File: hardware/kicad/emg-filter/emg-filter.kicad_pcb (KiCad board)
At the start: 4 copper layers, 50 x 40 mm, 84 parts, among them J1 Conn_01x02, J10 Conn_01x02, J11 Conn_01x02, J2 Conn_01x05, J3 Conn_01x02, J4 Conn_01x02, J5 Conn_01x02, J6 Conn_01x02, J7 Conn_01x02, J8 Conn_01x02, J9 Conn_01x02, U1 LM4565, U2 LM4565, U3 LM4565, U4 LM4565, U5 LM4565, U6 LM4565, U7 INA2332

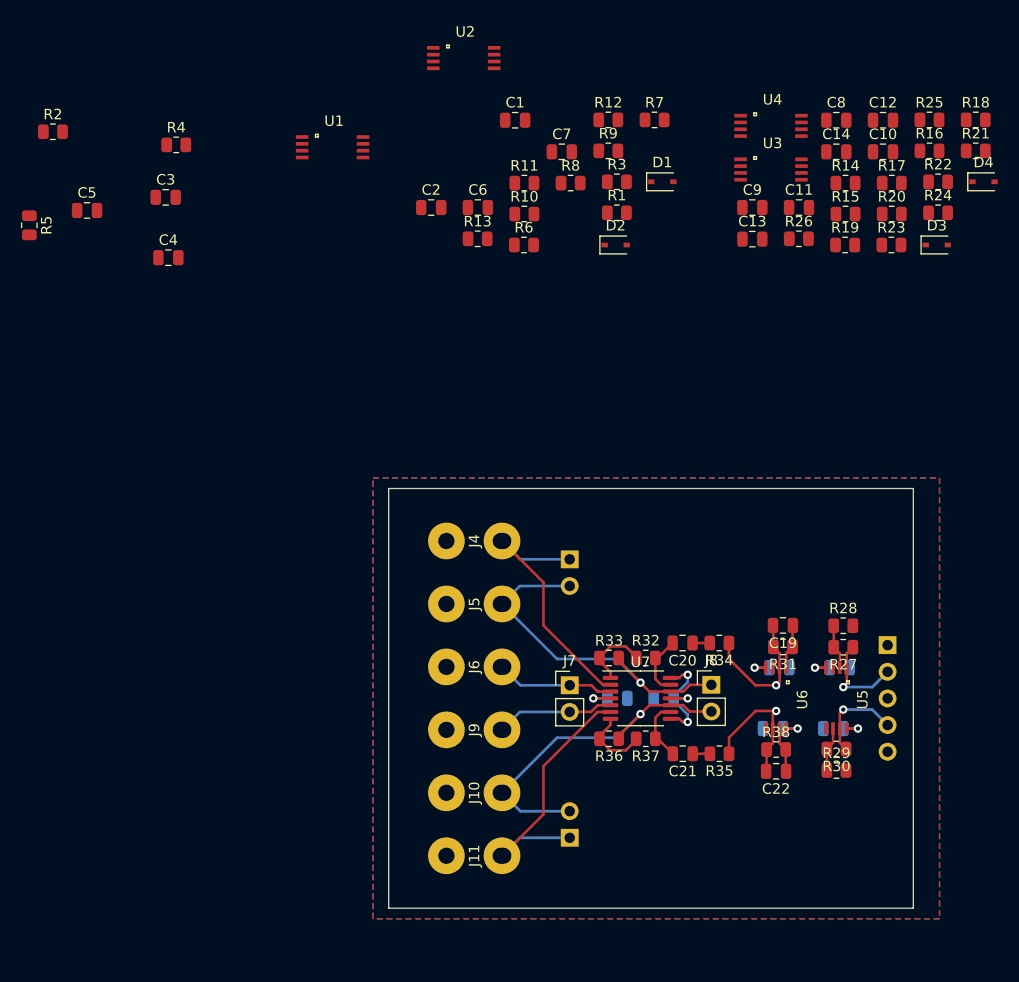
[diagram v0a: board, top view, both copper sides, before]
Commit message: Done - Ready for manufacturing
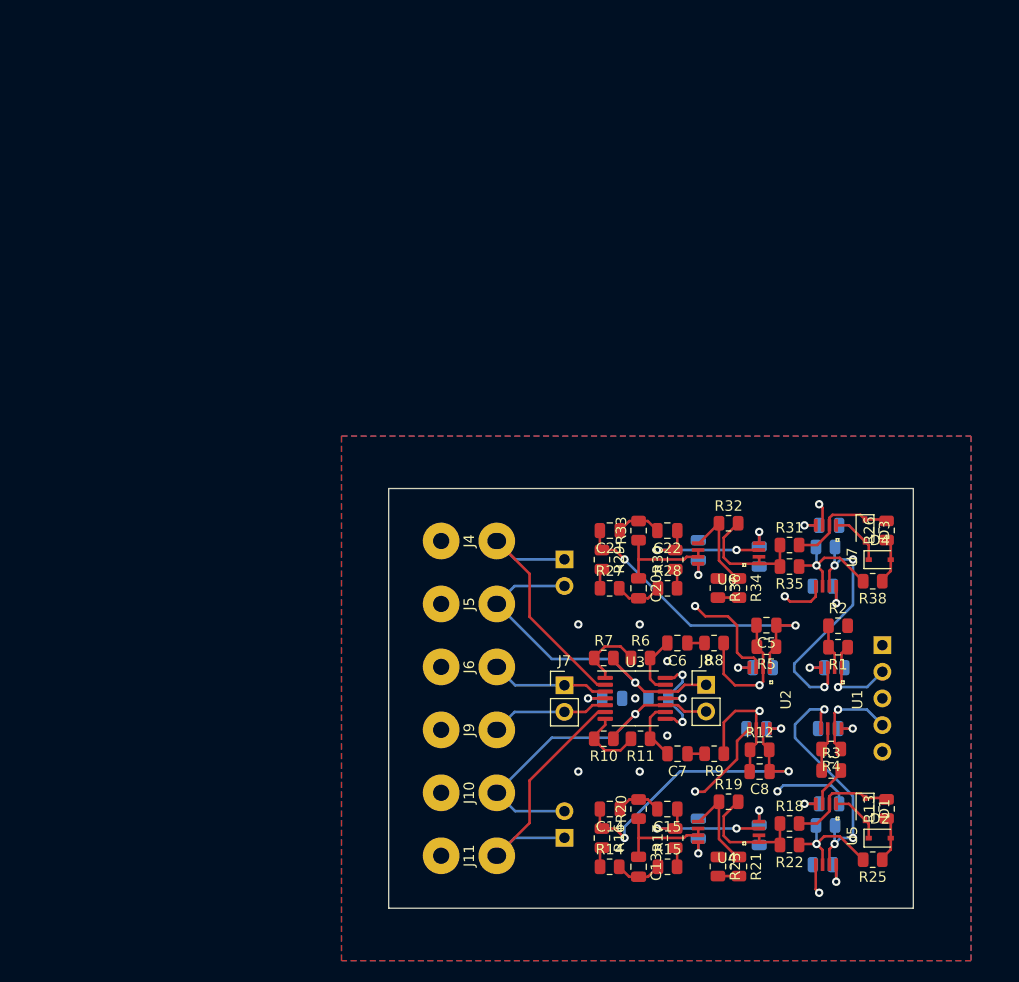
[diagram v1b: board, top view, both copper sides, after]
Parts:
- C1, C2, C9: moved to B.Cu
- C10, C3: value 20n -> 0.1u; moved to B.Cu
- C11, C12, C4: value 10n -> 0.1u; moved to B.Cu
- C13, C6, C7: value 0.1u -> 20n
- C14: value 0.1u -> 10n
- C15: value 0.1u -> 10n; moved to F.Cu
- C19: value 2n -> 0.1u; moved to B.Cu
- C21: value 20n -> 10n
- C22: value 2n -> 10n
- C5: value 10n -> 2n
- C8: value 0.1u -> 2n
- R11: value 133k -> 191k
- R12: value 10k -> 261k
- R13, R26: value 5k -> 10k
- R14, R27: value 10k -> 132k
- R15, R17: value 132k -> 133k
- R16: value 133k -> 132k
- R18, R22: value 133k -> 10k
- R19: value 10k -> 2k
- R2: value 132k -> 2k
- R20, R28: value 2k -> 133k
- R23, R30, R33, R36: value 10k -> 133k
- R24: value 133k -> 10k; moved to B.Cu
- R25: value 10k -> 5k
- R29: value 2k -> 132k
- R3: value 133k -> 2k
- R31, R35: value 261k -> 10k
- R32: value 191k -> 2k
- R34: value 261k -> 133k
- R37: value 191k -> 10k; moved to B.Cu
- R38: value 261k -> 5k
- R4: value 132k -> 10k
- R5, R8, R9: value 133k -> 261k
- R6: value 10k -> 191k
- R7: value 2k -> 10k
- U3: value LM4565 -> INA2332; footprint emg-filter:LM4565 -> Package_SO:TSSOP-14_4.4x5mm_P0.65mm
- U7: value INA2332 -> LM4565; footprint Package_SO:TSSOP-14_4.4x5mm_P0.65mm -> emg-filter:LM4565
- moved R2 88.4 mm to (92.3, 108.1)
- moved R4 84.9 mm to (91.7, 119.8), turned to 180 degrees
- moved R5 80.9 mm to (85.5, 110.1), turned to 180 degrees
- moved C5 75.9 mm to (85.5, 108.0), turned to 180 degrees
- moved R16 72.6 mm to (69.8, 128.3), turned to 270 degrees
- moved U1 72.1 mm to (92.7, 112.1), turned to 270 degrees
- moved R21 71.8 mm to (82.9, 131.0), turned to 270 degrees
- moved C4 71.8 mm to (84.5, 117.9), turned to 180 degrees
- moved C12 71.2 mm to (90.9, 130.8), turned to 180 degrees
- moved R25 70.7 mm to (95.6, 130.4), turned to 180 degrees
- moved R18 69.4 mm to (87.7, 126.9)
- moved U4 69.3 mm to (84.8, 128.7), turned to 180 degrees
- moved R14 68.9 mm to (70.6, 131.1)
- moved U2 67.2 mm to (85.8, 112.1), turned to 270 degrees
- moved C3 67.0 mm to (75.2, 115.0)
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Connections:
- C1 pad 1: +5V -> GND
- C1 pad 2: GND -> +5V
- C10 pad 1: Net-(C10-Pad1) -> GND
- C10 pad 2: Net-(C10-Pad2) -> -5V
- C11 pad 1: Net-(C11-Pad1) -> +5V
- C11 pad 2: /emg_module/sheet625420FA/BP_NOTCH -> GND
- C12 pad 1: Net-(C12-Pad1) -> +5V
- C12 pad 2: Net-(C11-Pad1) -> GND
- C13 pad 1: GND -> Net-(C13-Pad1)
- C13 pad 2: -5V -> Net-(C13-Pad2)
- C14 pad 1: -5V -> Net-(C14-Pad1)
- C14 pad 2: GND -> /emg_module/sheet625420F9/BP_NOTCH
- C15 pad 1: GND -> Net-(C15-Pad1)
- C15 pad 2: +5V -> Net-(C14-Pad1)
- C16 pad 1: -5V -> GND
- C16 pad 2: GND -> -5V
- C17 pad 1: GND -> -5V
- C17 pad 2: +5V -> GND
- C19 pad 1: /emg_module/sheet625420FA/BP_NOTCH -> +5V
- C19 pad 2: Net-(C19-Pad2) -> GND
- C2 pad 1: +5V -> -5V
- C21 pad 2: Net-(C21-Pad2) -> /emg_module/sheet625420FA/BP_NOTCH
- C22 pad 1: /emg_module/sheet625420F9/BP_NOTCH -> Net-(C22-Pad1)
- C22 pad 2: Net-(C22-Pad2) -> Net-(C21-Pad1)
- C24 pad 1: GND -> -5V
- C24 pad 2: -5V -> GND
- C3 pad 1: Net-(C3-Pad1) -> GND
- C3 pad 2: Net-(C3-Pad2) -> +5V
- C4 pad 1: Net-(C4-Pad1) -> +5V
- C4 pad 2: /emg_module/sheet625420F9/BP_NOTCH -> GND
- C5 pad 1: Net-(C5-Pad1) -> /emg_module/sheet625420FA/BP_NOTCH
- C5 pad 2: Net-(C4-Pad1) -> Net-(C5-Pad2)
- C6 pad 1: GND -> Net-(C6-Pad1)
- C6 pad 2: -5V -> Net-(C6-Pad2)
- C7 pad 1: -5V -> Net-(C7-Pad1)
- C7 pad 2: GND -> Net-(C7-Pad2)
- C8 pad 1: +5V -> /emg_module/sheet625420F9/BP_NOTCH
- C8 pad 2: GND -> Net-(C8-Pad2)
- C9 pad 1: +5V -> GND
- C9 pad 2: GND -> -5V
- R1 pad 1: Net-(D2-Pad2) -> /emg_module/OUT_A
- R1 pad 2: Net-(D1-Pad1) -> Net-(R1-Pad2)
- R10 pad 1: Net-(R10-Pad1) -> /emg_module/REF_B
- R11 pad 1: GND -> Net-(C7-Pad2)
- R11 pad 2: Net-(R11-Pad2) -> Net-(R10-Pad2)
- R12 pad 1: /emg_module/sheet625420F9/RECT_AMP -> Net-(C8-Pad2)
- R12 pad 2: Net-(R10-Pad1) -> /emg_module/sheet625420F9/BP_NOTCH
- R13 pad 2: Net-(R10-Pad1) -> Net-(D1-Pad1)
- R14 pad 1: Net-(D4-Pad2) -> Net-(R14-Pad1)
- R14 pad 2: Net-(D3-Pad1) -> Net-(C13-Pad2)
- R15 pad 1: Net-(R15-Pad1) -> Net-(C13-Pad2)
- R15 pad 2: Net-(C10-Pad2) -> Net-(R15-Pad2)
- R16 pad 1: Net-(C10-Pad2) -> /emg_module/sheet625420F9/BP_NOTCH
- R16 pad 2: Net-(R16-Pad2) -> Net-(R14-Pad1)
- R17 pad 1: /emg_module/sheet625420FA/BP_NOTCH -> Net-(R15-Pad2)
- R17 pad 2: Net-(R15-Pad1) -> Net-(C15-Pad1)
- R18 pad 1: Net-(R16-Pad2) -> Net-(R18-Pad1)
- R18 pad 2: Net-(C12-Pad1) -> Net-(D1-Pad1)
- R19 pad 2: Net-(D3-Pad1) -> Net-(R18-Pad1)
- R2 pad 1: Net-(R2-Pad1) -> Net-(R1-Pad2)
- R2 pad 2: Net-(C3-Pad2) -> GND
- R20 pad 1: Net-(R20-Pad1) -> Net-(C13-Pad1)
- R20 pad 2: Net-(R19-Pad1) -> Net-(C14-Pad1)
- R21 pad 1: Net-(C10-Pad1) -> Net-(R19-Pad1)
- R21 pad 2: Net-(C11-Pad1) -> Net-(R21-Pad2)
- R22 pad 1: Net-(R20-Pad1) -> Net-(R22-Pad1)
- R22 pad 2: Net-(R22-Pad2) -> Net-(R18-Pad1)
- R23 pad 1: Net-(R23-Pad1) -> GND
- R23 pad 2: Net-(R19-Pad1) -> Net-(R21-Pad2)
- R24 pad 1: GND -> /emg_module/sheet625420F9/RECT_AMP
- R24 pad 2: Net-(R22-Pad2) -> Net-(R22-Pad1)
- R25 pad 1: /emg_module/sheet625420FA/RECT_AMP -> Net-(D2-Pad2)
- R25 pad 2: Net-(R23-Pad1) -> Net-(R22-Pad1)
- R26 pad 2: Net-(R23-Pad1) -> Net-(D3-Pad1)
- R27 pad 1: /emg_module/OUT_A -> Net-(R27-Pad1)
- R27 pad 2: Net-(R27-Pad2) -> Net-(C20-Pad2)
- R28 pad 1: Net-(R27-Pad2) -> Net-(C20-Pad2)
- R28 pad 2: GND -> Net-(R28-Pad2)
- R29 pad 1: Net-(R29-Pad1) -> /emg_module/sheet625420FA/BP_NOTCH
- R29 pad 2: GND -> Net-(R27-Pad1)
- R3 pad 1: Net-(C3-Pad2) -> Net-(R3-Pad1)
- R3 pad 2: Net-(R3-Pad2) -> GND
- R30 pad 1: /emg_module/OUT_B -> Net-(R28-Pad2)
- R30 pad 2: Net-(R29-Pad1) -> Net-(C22-Pad1)
- R31 pad 1: /emg_module/sheet625420FA/BP_NOTCH -> Net-(R31-Pad1)
- R31 pad 2: Net-(C19-Pad2) -> Net-(D3-Pad1)
- R32 pad 2: Net-(C20-Pad2) -> Net-(R31-Pad1)
- R33 pad 1: Net-(R32-Pad1) -> Net-(C20-Pad1)
- R33 pad 2: /emg_module/REF_A -> Net-(C21-Pad1)
- R34 pad 1: Net-(C19-Pad2) -> Net-(R32-Pad1)
- R34 pad 2: Net-(C20-Pad1) -> Net-(R34-Pad2)
- R35 pad 1: Net-(C22-Pad2) -> Net-(R35-Pad1)
- R35 pad 2: Net-(C21-Pad1) -> Net-(R31-Pad1)
- R36 pad 1: /emg_module/REF_B -> GND
- R36 pad 2: Net-(R36-Pad2) -> Net-(R34-Pad2)
- R37 pad 1: Net-(C21-Pad2) -> /emg_module/sheet625420FA/RECT_AMP
- R37 pad 2: Net-(R36-Pad2) -> Net-(R35-Pad1)
- R38 pad 1: Net-(C22-Pad2) -> Net-(D4-Pad2)
- R38 pad 2: /emg_module/sheet625420F9/BP_NOTCH -> Net-(R35-Pad1)
- R4 pad 1: /emg_module/sheet625420F9/BP_NOTCH -> /emg_module/OUT_B
- R4 pad 2: Net-(R2-Pad1) -> Net-(R3-Pad1)
- R5 pad 1: Net-(R3-Pad2) -> /emg_module/sheet625420FA/BP_NOTCH
- R5 pad 2: Net-(C5-Pad1) -> Net-(C5-Pad2)
- R6 pad 1: Net-(R10-Pad2) -> Net-(R6-Pad1)
- R6 pad 2: Net-(D1-Pad1) -> Net-(C6-Pad2)
- R7 pad 1: Net-(R7-Pad1) -> Net-(R6-Pad1)
- R7 pad 2: Net-(R10-Pad2) -> /emg_module/REF_A
- R8 pad 1: Net-(C3-Pad1) -> Net-(C5-Pad2)
- R8 pad 2: Net-(C4-Pad1) -> Net-(C6-Pad1)
- R9 pad 1: Net-(R7-Pad1) -> Net-(C8-Pad2)
- R9 pad 2: Net-(R11-Pad2) -> Net-(C7-Pad1)
- U1 pad 1: Net-(R10-Pad2) -> /emg_module/OUT_A
- U1 pad 2: Net-(R10-Pad2) -> Net-(R1-Pad2)
- U1 pad 3: Net-(C5-Pad1) -> /emg_module/sheet625420FA/RECT_AMP
- U1 pad 5: Net-(R7-Pad1) -> /emg_module/sheet625420F9/RECT_AMP
- U1 pad 6: Net-(C3-Pad1) -> Net-(R3-Pad1)
- U1 pad 7: Net-(C3-Pad1) -> /emg_module/OUT_B
- U2 pad 1: Net-(D1-Pad2) -> /emg_module/sheet625420FA/BP_NOTCH
- U2 pad 2: Net-(D1-Pad1) -> Net-(C5-Pad2)
- U2 pad 6: Net-(R10-Pad1) -> Net-(C8-Pad2)
- U2 pad 7: /emg_module/sheet625420F9/RECT_AMP -> /emg_module/sheet625420F9/BP_NOTCH
- U3 pad 1: Net-(R19-Pad1) -> Net-(R6-Pad1)
- U3 pad 2: Net-(R19-Pad1) -> /emg_module/VIN_A
- U3 pad 3: Net-(C12-Pad1) -> /emg_module/sheet625420FD/+VIN_A_INA
- U3 pad 5: Net-(R20-Pad1) -> /emg_module/sheet625420FC/+VIN_B_INA
- U3 pad 6: Net-(C10-Pad1) -> /emg_module/VIN_B
- U3 pad 7: Net-(C10-Pad1) -> Net-(R10-Pad2)
- U4 pad 1: Net-(D3-Pad2) -> Net-(R18-Pad1)
- U4 pad 2: Net-(D3-Pad1) -> Net-(R18-Pad1)
- U4 pad 3: GND -> Net-(C15-Pad1)
- U4 pad 5: GND -> Net-(R19-Pad1)
- U4 pad 6: Net-(R23-Pad1) -> Net-(C13-Pad1)
- U4 pad 7: /emg_module/sheet625420FA/RECT_AMP -> Net-(C13-Pad1)
- U5 pad 1: /emg_module/OUT_A -> Net-(D1-Pad2)
- U5 pad 2: Net-(R27-Pad2) -> Net-(D1-Pad1)
- U5 pad 3: /emg_module/sheet625420FA/RECT_AMP -> GND
- U5 pad 5: /emg_module/sheet625420F9/RECT_AMP -> GND
- U5 pad 6: Net-(R29-Pad1) -> Net-(R22-Pad1)
- U5 pad 7: /emg_module/OUT_B -> /emg_module/sheet625420F9/RECT_AMP
- U6 pad 1: /emg_module/sheet625420FA/BP_NOTCH -> Net-(R31-Pad1)
- U6 pad 2: Net-(C19-Pad2) -> Net-(R31-Pad1)
- U6 pad 3: GND -> Net-(C22-Pad1)
- U6 pad 5: GND -> Net-(R32-Pad1)
- U6 pad 6: Net-(C22-Pad2) -> Net-(C20-Pad1)
- U6 pad 7: /emg_module/sheet625420F9/BP_NOTCH -> Net-(C20-Pad1)
- U7 pad 1: Net-(R32-Pad1) -> Net-(D3-Pad2)
- U7 pad 2: /emg_module/VIN_A -> Net-(D3-Pad1)
- U7 pad 3: /emg_module/sheet625420FD/+VIN_A_INA -> GND
- U7 pad 5: /emg_module/sheet625420FC/+VIN_B_INA -> GND
- U7 pad 6: /emg_module/VIN_B -> Net-(R35-Pad1)
- U7 pad 7: Net-(R36-Pad2) -> /emg_module/sheet625420FA/RECT_AMP
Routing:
- net GND: track 0.00 -> 39.2 mm, vias 0 -> 13
- net /emg_module/sheet625420FA/BP_NOTCH: track 4.28 -> 29.5 mm, vias 0 -> 2
- net /emg_module/sheet625420F9/BP_NOTCH: track 4.33 -> 29.5 mm, vias 0 -> 2
- net /emg_module/sheet625420FA/RECT_AMP: track 0.00 -> 24.6 mm, vias 0 -> 3
- net /emg_module/sheet625420F9/RECT_AMP: track 0.00 -> 24.6 mm, vias 0 -> 3
- net Net-(C15-Pad1): track 0.00 -> 13.4 mm, vias 0 -> 2
- net Net-(C22-Pad1): track 0.00 -> 13.4 mm, vias 0 -> 2
- net Net-(C22-Pad2): track 13.2 -> 0.00 mm, vias 1 -> 0
- net Net-(C19-Pad2): track 13.1 -> 0.00 mm, vias 1 -> 0
- net Net-(C8-Pad2): track 0.00 -> 13.0 mm, vias 0 -> 1
- net Net-(C5-Pad2): track 0.00 -> 12.9 mm, vias 0 -> 1
- net Net-(R31-Pad1): track 0.00 -> 12.2 mm
- net Net-(R18-Pad1): track 0.00 -> 12.2 mm
- net +5V: track 17.6 -> 29.3 mm, vias 5 -> 9
- net Net-(R35-Pad1): track 0.00 -> 11.5 mm, vias 0 -> 1
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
